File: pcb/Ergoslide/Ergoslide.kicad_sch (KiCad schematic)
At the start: 204 parts, among them J1 Conn_01x02_Socket, J2 Conn_01x02_Socket, SW1 Switch, SW2 Power Switch

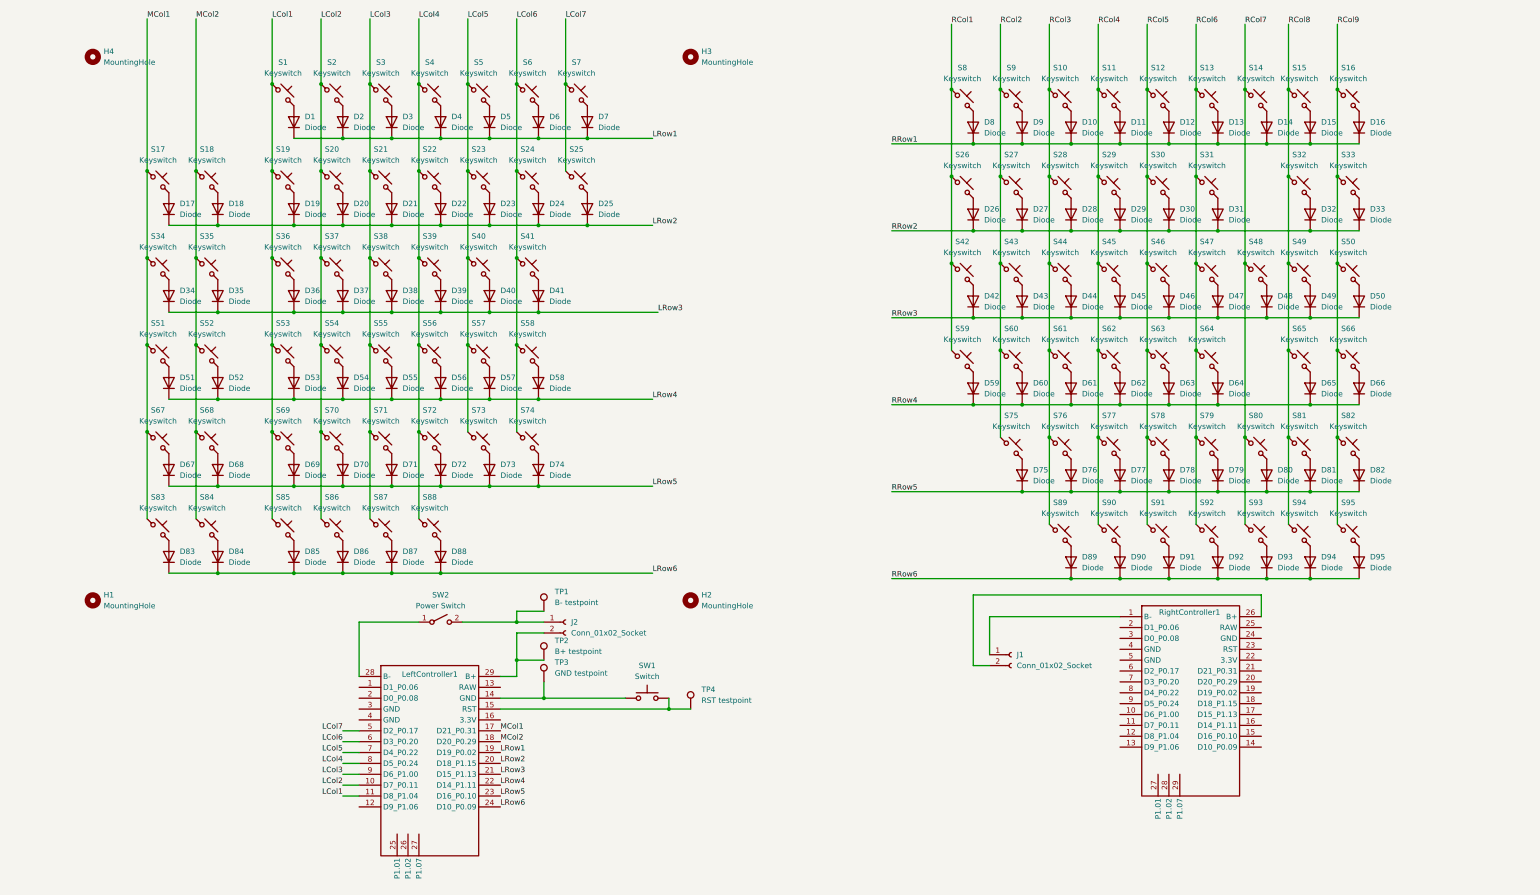
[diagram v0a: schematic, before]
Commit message: Add TL3330AF260GQ to the PCB, start wiring up the second half
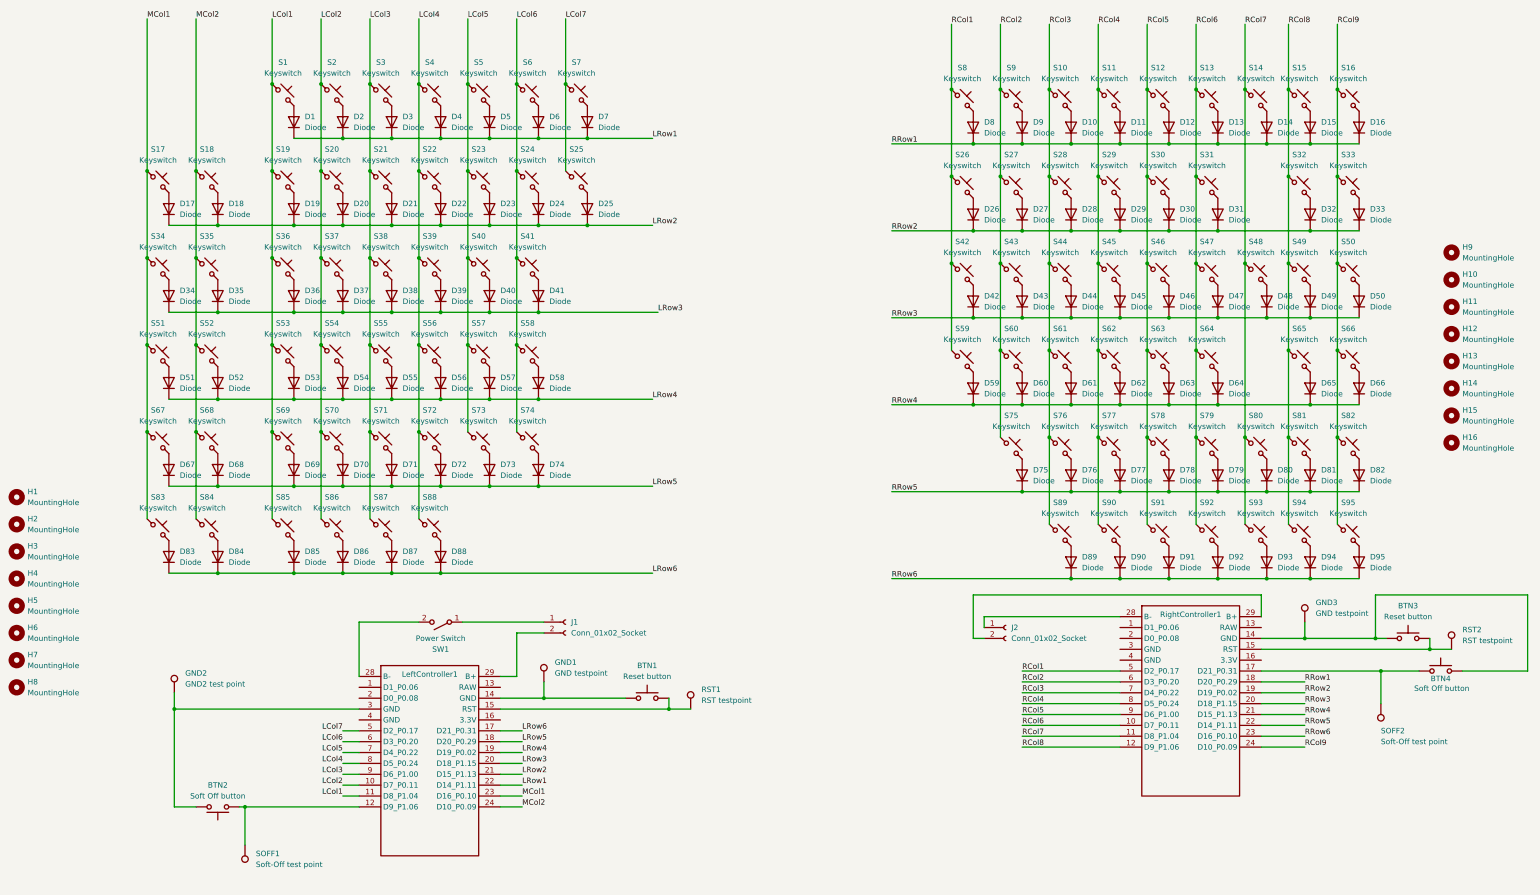
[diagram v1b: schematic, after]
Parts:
- removed TP1: B- testpoint, TestPoint:TestPoint_Pad_2.0x2.0mm, symbol Connector:TestPoint
- removed TP2: B+ testpoint, TestPoint:TestPoint_Pad_2.0x2.0mm, symbol Connector:TestPoint
- added BTN2, BTN4: Soft Off button, TL3330AF260QG:SW_TL3330AF260QG, symbol ScottoKeebs:Placeholder_Switch
- added BTN3: Reset button, TL3330AF260QG:SW_TL3330AF260QG, symbol ScottoKeebs:Placeholder_Switch
- added GND2: GND2 test point, TestPoint:TestPoint_Pad_2.0x2.0mm, symbol Connector:TestPoint
- added GND3: GND testpoint, TestPoint:TestPoint_Pad_2.0x2.0mm, symbol Connector:TestPoint
- added H10, H11, H12, H13, H14, H15, H16, H5, H6, H7, H8, H9: MountingHole, MountingHole:MountingHole_2.2mm_M2, symbol Mechanical:MountingHole
- added RST1, RST2: RST testpoint, TestPoint:TestPoint_Pad_2.0x2.0mm, symbol Connector:TestPoint
- added SOFF2: Soft-Off test point, TestPoint:TestPoint_Pad_2.0x2.0mm, symbol Connector:TestPoint
- BTN1: renamed from SW1; value Switch -> Reset button; footprint Button_Switch_SMD:Panasonic_EVQPUL_EVQPUC -> TL3330AF260QG:SW_TL3330AF260QG
- RightController1: footprint supermini-nrf52840-kicad:SuperMini NRF52840 -> supermini-nrf52840-kicad:SimpleMini NRF52840
- SOFF1: renamed from TP4; value RST testpoint -> Soft-Off test point
- SW1: renamed from SW2; footprint ScottoKeebs_Components:Switch_SSAL220100 -> Button_Switch_SMD:SW_SPDT_CK_JS102011SAQN
- renumbered TP3 to GND1, H4 to H1, H3 to H2, H1 to H3, H2 to H4, J2 to J1, J1 to J2
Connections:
- net LRow1: now also LeftController1.22 (D14_P1.11); no longer LeftController1.19 (D19_P0.02)
- net LRow2: now also LeftController1.21 (D15_P1.13); no longer LeftController1.20 (D18_P1.15)
- net LRow3: now also LeftController1.20 (D18_P1.15); no longer LeftController1.21 (D15_P1.13)
- net LRow4: now also LeftController1.19 (D19_P0.02); no longer LeftController1.22 (D14_P1.11)
- net LRow5: now also LeftController1.18 (D20_P0.29); no longer LeftController1.23 (D16_P0.10)
- net LRow6: now also LeftController1.17 (D21_P0.31); no longer LeftController1.24 (D10_P0.09)
- net MCol1: now also LeftController1.23 (D16_P0.10); no longer LeftController1.17 (D21_P0.31)
- net MCol2: now also LeftController1.24 (D10_P0.09); no longer LeftController1.18 (D20_P0.29)
- net RCol1: now also RightController1.5 (D2_P0.17)
- net RCol2: now also RightController1.6 (D3_P0.20)
- net RCol3: now also RightController1.7 (D4_P0.22)
- net RCol4: now also RightController1.8 (D5_P0.24)
- net RCol5: now also RightController1.9 (D6_P1.00)
- net RCol6: now also RightController1.10 (D7_P0.11)
- net RCol7: now also RightController1.11 (D8_P1.04)
- net RCol8: now also RightController1.12 (D9_P1.06)
- net RCol9: now also RightController1.24 (D10_P0.09)
- net RRow1: now also RightController1.18 (D20_P0.29)
- net RRow2: now also RightController1.19 (D19_P0.02)
- net RRow3: now also RightController1.20 (D18_P1.15)
- net RRow4: now also RightController1.21 (D15_P1.13)
- net RRow5: now also RightController1.22 (D14_P1.11)
- net RRow6: now also RightController1.23 (D16_P0.10)
- net at SW1.1 (A): now also J1.1 (Pin_1); no longer LeftController1.28 (B-)
- net at SW1.2 (B): now also LeftController1.28 (B-); no longer J1.1 (Pin_1)
- net at BTN1.2, LeftController1.15 (RST): now also RST1.1; no longer SOFF1.1
- net at RightController1.1 (D1_P0.06): no longer J2.1 (Pin_1)
- net at J2.2 (Pin_2): now also RightController1.29 (B+); no longer RightController1.26 (B+)
- net at RightController1.14 (GND): now also BTN3.1, BTN4.2, GND3.1
- net at RightController1.15 (RST): now also BTN3.2, RST2.1
- net at RightController1.17 (D21_P0.31): now also BTN4.1, SOFF2.1
- net at RightController1.28 (B-): now also J2.1 (Pin_1)
- net at LeftController1.12 (D9_P1.06): now also SOFF1.1, BTN2.1
- net at LeftController1.3 (GND): now also BTN2.2, GND2.1
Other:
- moved on the sheet: H1, H2, H3, H4, J2, SOFF1, SW1
